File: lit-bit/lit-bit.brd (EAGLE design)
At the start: 71 parts, among them J2 USB_MICRO_B_SMD_FEMALE, J3 ISP, U2 32U4, U3 73831, U4 ADXL345, U5 S-1335, U6 MCP7940N, U7 24FC1025, Y1 8MHz, Y2 32.768kHz, Y3 32.768kHz, Y4 16MHz

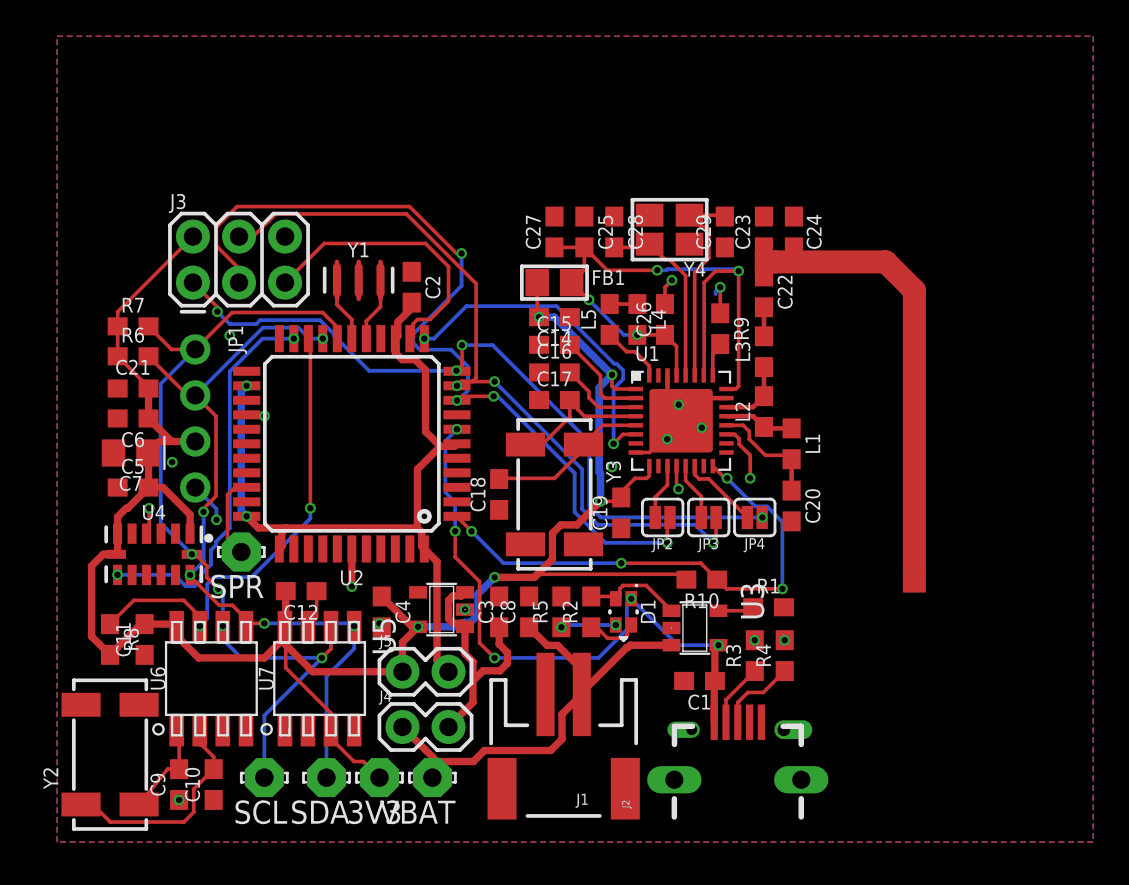
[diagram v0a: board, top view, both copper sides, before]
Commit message: finally have something decent
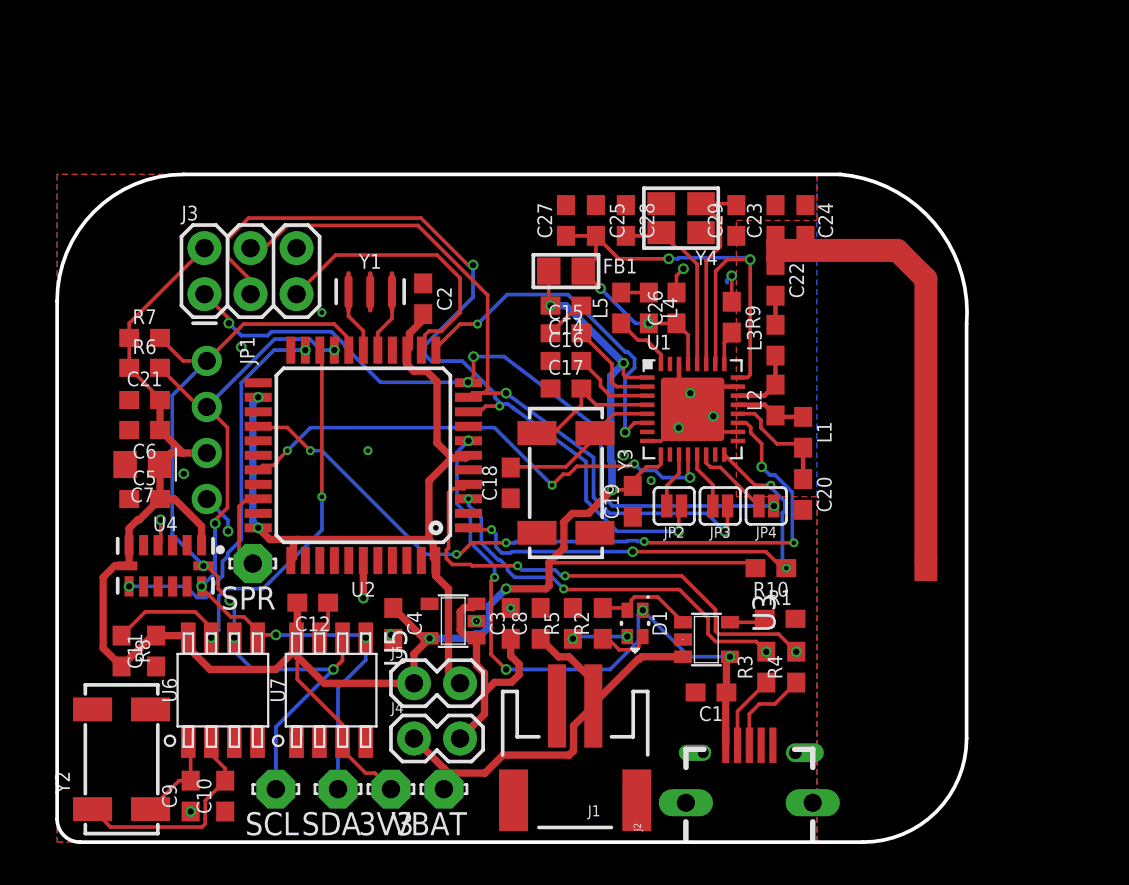
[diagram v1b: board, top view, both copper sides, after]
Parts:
- moved R10 3.86 mm to (39.4, 15.1)
- moved J2 1.42 mm to (41.9, 0.00)
- moved Y4 0.90 mm to (34.4, 34.4)
- moved L1 0.90 mm to (41.1, 22.6)
- moved L2 0.90 mm to (39.6, 24.4)
- moved L3 0.90 mm to (39.6, 27.7)
- moved R4 0.90 mm to (40.8, 9.65)
- moved C14 0.90 mm to (28.1, 29.6)
- moved C15 0.90 mm to (28.1, 28.1)
- moved Y3 0.90 mm to (28.1, 19.8)
- moved C20 0.90 mm to (41.1, 19.2)
- moved C22 0.90 mm to (39.6, 31.0)
- moved C23 0.90 mm to (39.6, 34.3)
- moved C29 0.90 mm to (37.5, 34.3)
- moved L4 0.90 mm to (32.6, 29.5)
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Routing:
- net NRF-RST: track 4.25 -> 41.2 mm, vias 2 -> 6
- net D+: track 0.00 -> 27.1 mm, vias 1 -> 3
- net REQN: track 1.31 -> 28.3 mm, vias 1 -> 4
- net N$6: track 0.00 -> 21.5 mm, vias 1 -> 3
- net GND: track 20.6 -> 25.5 mm, vias 14 -> 18
- net 3V3: track 116.9 -> 121.3 mm
- net RDYN: track 28.4 -> 27.3 mm
- net SCK: track 48.4 -> 47.5 mm, vias 4 -> 3
- net MISO: track 41.1 -> 40.2 mm
- net MOSI: track 42.6 -> 41.7 mm, vias 3 -> 2
- net VUSB: track 34.0 -> 34.8 mm
- net UD+: track 4.39 -> 5.03 mm
- net UD-: track 3.48 -> 4.11 mm
- net N$21: track 12.1 -> 12.7 mm
- net ACTIVE: track 18.9 -> 19.5 mm
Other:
- board outline added: 50.2 x 36.8 mm
